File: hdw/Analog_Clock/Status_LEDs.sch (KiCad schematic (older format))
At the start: 35 parts

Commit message: More schematic work
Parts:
- removed U? (x7): 74LVC1G97, Package_TO_SOT_SMD:SOT-363_SC-70-6, symbol Custom_Library:74LVC1G97_Power_NOT
- added U? (x7): 74LVC1G06, TO_SOT_Packages_SMD:SOT-353_SC-70-5, symbol Custom_Library:74LVC1G06_Power
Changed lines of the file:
@@
 EESchema Schematic File Version 4
+LIBS:Analog_Clock-cache
 EELAYER 30 0
 EELAYER END
@@
 $EndComp
 $Comp
-L Custom_Library:74LVC1G97_Power_NOT U?
-U 1 1 5E499235
+L Custom_Library:74LVC1G06_Power U?
+U 1 1 5E9D80F8
 P 2400 2220
-F 0 "U?" H 2460 2370 50  0000 L CNN
-F 1 "74LVC1G97" H 2460 2070 50  0000 L CNN
-F 2 "Package_TO_SOT_SMD:SOT-363_SC-70-6" H 2450 2220 50  0001 C CNN
-F 3 "http://www.ti.com/lit/ds/symlink/sn74lvc1g97.pdf" H 2450 2220 50  0001 C CNN
-F 4 "296-15582-1-ND" H 2400 2220 50  0001 C CNN "Digi-Key PN"
+F 0 "U?" H 2500 2370 50  0000 L CNN
+F 1 "74LVC1G06" H 2500 2120 50  0000 L CNN
+F 2 "TO_SOT_Packages_SMD:SOT-353_SC-70-5" H 2400 2270 50  0001 C CNN
+F 3 "http://www.ti.com/lit/ds/symlink/sn74lvc1g06.pdf" H 2400 2220 50  0001 C CNN
+F 4 "296-8484-1-ND" H 2400 2220 50  0001 C CNN "Digi-Key PN"
 	1    2400 2220
 	1    0    0    -1
 $EndComp
 $Comp
-L Custom_Library:74LVC1G97_Power_NOT U?
-U 1 1 5E499F9B
+L Custom_Library:74LVC1G06_Power U?
+U 1 1 5E9DA040
 P 4400 2220
-F 0 "U?" H 4460 2370 50  0000 L CNN
-F 1 "74LVC1G97" H 4460 2070 50  0000 L CNN
-F 2 "Package_TO_SOT_SMD:SOT-363_SC-70-6" H 4450 2220 50  0001 C CNN
-F 3 "http://www.ti.com/lit/ds/symlink/sn74lvc1g97.pdf" H 4450 2220 50  0001 C CNN
-F 4 "296-15582-1-ND" H 4400 2220 50  0001 C CNN "Digi-Key PN"
+F 0 "U?" H 4500 2370 50  0000 L CNN
+F 1 "74LVC1G06" H 4500 2120 50  0000 L CNN
+F 2 "TO_SOT_Packages_SMD:SOT-353_SC-70-5" H 4400 2270 50  0001 C CNN
+F 3 "http://www.ti.com/lit/ds/symlink/sn74lvc1g06.pdf" H 4400 2220 50  0001 C CNN
+F 4 "296-8484-1-ND" H 4400 2220 50  0001 C CNN "Digi-Key PN"
 	1    4400 2220
 	1    0    0    -1
 $EndComp
 $Comp
-L Custom_Library:74LVC1G97_Power_NOT U?
-U 1 1 5E49A9B3
+L Custom_Library:74LVC1G06_Power U?
+U 1 1 5E9DA915
 P 6400 2220
-F 0 "U?" H 6460 2370 50  0000 L CNN
-F 1 "74LVC1G97" H 6460 2070 50  0000 L CNN
-F 2 "Package_TO_SOT_SMD:SOT-363_SC-70-6" H 6450 2220 50  0001 C CNN
-F 3 "http://www.ti.com/lit/ds/symlink/sn74lvc1g97.pdf" H 6450 2220 50  0001 C CNN
-F 4 "296-15582-1-ND" H 6400 2220 50  0001 C CNN "Digi-Key PN"
+F 0 "U?" H 6500 2370 50  0000 L CNN
+F 1 "74LVC1G06" H 6500 2120 50  0000 L CNN
+F 2 "TO_SOT_Packages_SMD:SOT-353_SC-70-5" H 6400 2270 50  0001 C CNN
+F 3 "http://www.ti.com/lit/ds/symlink/sn74lvc1g06.pdf" H 6400 2220 50  0001 C CNN
+F 4 "296-8484-1-ND" H 6400 2220 50  0001 C CNN "Digi-Key PN"
 	1    6400 2220
 	1    0    0    -1
 $EndComp
 $Comp
-L Custom_Library:74LVC1G97_Power_NOT U?
-U 1 1 5E49B430
+L Custom_Library:74LVC1G06_Power U?
+U 1 1 5E9DB45A
 P 8400 2220
-F 0 "U?" H 8460 2370 50  0000 L CNN
-F 1 "74LVC1G97" H 8460 2070 50  0000 L CNN
-F 2 "Package_TO_SOT_SMD:SOT-363_SC-70-6" H 8450 2220 50  0001 C CNN
-F 3 "http://www.ti.com/lit/ds/symlink/sn74lvc1g97.pdf" H 8450 2220 50  0001 C CNN
-F 4 "296-15582-1-ND" H 8400 2220 50  0001 C CNN "Digi-Key PN"
+F 0 "U?" H 8500 2370 50  0000 L CNN
+F 1 "74LVC1G06" H 8500 2120 50  0000 L CNN
+F 2 "TO_SOT_Packages_SMD:SOT-353_SC-70-5" H 8400 2270 50  0001 C CNN
+F 3 "http://www.ti.com/lit/ds/symlink/sn74lvc1g06.pdf" H 8400 2220 50  0001 C CNN
+F 4 "296-8484-1-ND" H 8400 2220 50  0001 C CNN "Digi-Key PN"
 	1    8400 2220
 	1    0    0    -1
 $EndComp
 $Comp
-L Custom_Library:74LVC1G97_Power_NOT U?
-U 1 1 5E49BF58
+L Custom_Library:74LVC1G06_Power U?
+U 1 1 5E9DBF5D
 P 6400 4220
-F 0 "U?" H 6460 4370 50  0000 L CNN
-F 1 "74LVC1G97" H 6460 4070 50  0000 L CNN
-F 2 "Package_TO_SOT_SMD:SOT-363_SC-70-6" H 6450 4220 50  0001 C CNN
-F 3 "http://www.ti.com/lit/ds/symlink/sn74lvc1g97.pdf" H 6450 4220 50  0001 C CNN
-F 4 "296-15582-1-ND" H 6400 4220 50  0001 C CNN "Digi-Key PN"
+F 0 "U?" H 6500 4370 50  0000 L CNN
+F 1 "74LVC1G06" H 6500 4120 50  0000 L CNN
+F 2 "TO_SOT_Packages_SMD:SOT-353_SC-70-5" H 6400 4270 50  0001 C CNN
+F 3 "http://www.ti.com/lit/ds/symlink/sn74lvc1g06.pdf" H 6400 4220 50  0001 C CNN
+F 4 "296-8484-1-ND" H 6400 4220 50  0001 C CNN "Digi-Key PN"
 	1    6400 4220
 	1    0    0    -1
 $EndComp
 $Comp
-L Custom_Library:74LVC1G97_Power_NOT U?
-U 1 1 5E49CDEC
+L Custom_Library:74LVC1G06_Power U?
+U 1 1 5E9DCA66
 P 4400 4220
-F 0 "U?" H 4460 4370 50  0000 L CNN
-F 1 "74LVC1G97" H 4460 4070 50  0000 L CNN
-F 2 "Package_TO_SOT_SMD:SOT-363_SC-70-6" H 4450 4220 50  0001 C CNN
-F 3 "http://www.ti.com/lit/ds/symlink/sn74lvc1g97.pdf" H 4450 4220 50  0001 C CNN
-F 4 "296-15582-1-ND" H 4400 4220 50  0001 C CNN "Digi-Key PN"
+F 0 "U?" H 4500 4370 50  0000 L CNN
+F 1 "74LVC1G06" H 4500 4120 50  0000 L CNN
+F 2 "TO_SOT_Packages_SMD:SOT-353_SC-70-5" H 4400 4270 50  0001 C CNN
+F 3 "http://www.ti.com/lit/ds/symlink/sn74lvc1g06.pdf" H 4400 4220 50  0001 C CNN
+F 4 "296-8484-1-ND" H 4400 4220 50  0001 C CNN "Digi-Key PN"
 	1    4400 4220
 	1    0    0    -1
 $EndComp
 $Comp
-L Custom_Library:74LVC1G97_Power_NOT U?
-U 1 1 5E49D6D6
+L Custom_Library:74LVC1G06_Power U?
+U 1 1 5E9DD4E5
 P 2400 4220
-F 0 "U?" H 2460 4370 50  0000 L CNN
-F 1 "74LVC1G97" H 2460 4070 50  0000 L CNN
-F 2 "Package_TO_SOT_SMD:SOT-363_SC-70-6" H 2450 4220 50  0001 C CNN
-F 3 "http://www.ti.com/lit/ds/symlink/sn74lvc1g97.pdf" H 2450 4220 50  0001 C CNN
-F 4 "296-15582-1-ND" H 2400 4220 50  0001 C CNN "Digi-Key PN"
+F 0 "U?" H 2500 4370 50  0000 L CNN
+F 1 "74LVC1G06" H 2500 4120 50  0000 L CNN
+F 2 "TO_SOT_Packages_SMD:SOT-353_SC-70-5" H 2400 4270 50  0001 C CNN
+F 3 "http://www.ti.com/lit/ds/symlink/sn74lvc1g06.pdf" H 2400 4220 50  0001 C CNN
+F 4 "296-8484-1-ND" H 2400 4220 50  0001 C CNN "Digi-Key PN"
 	1    2400 4220
 	1    0    0    -1

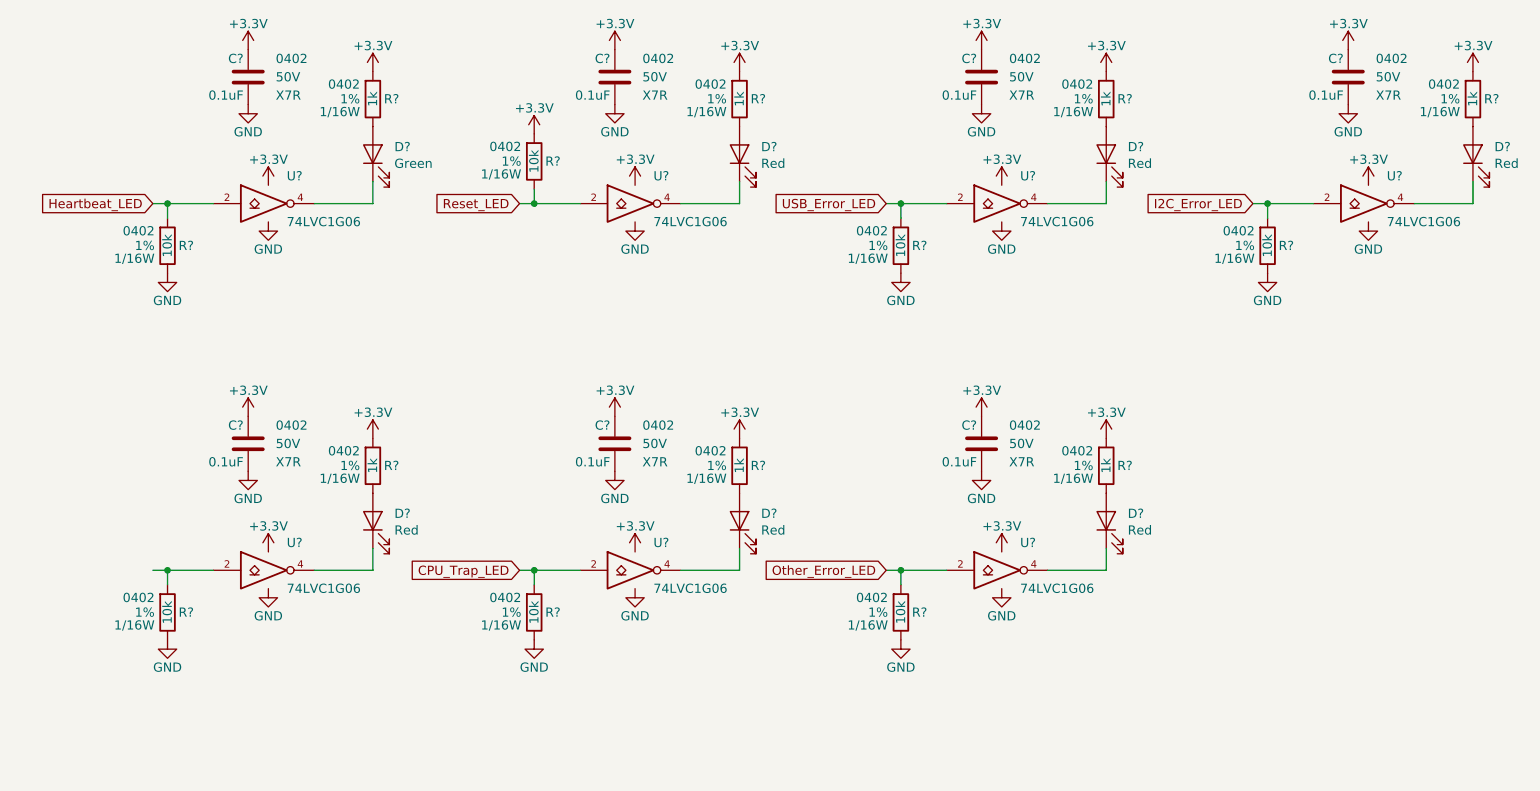
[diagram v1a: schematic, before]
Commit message: More sch work
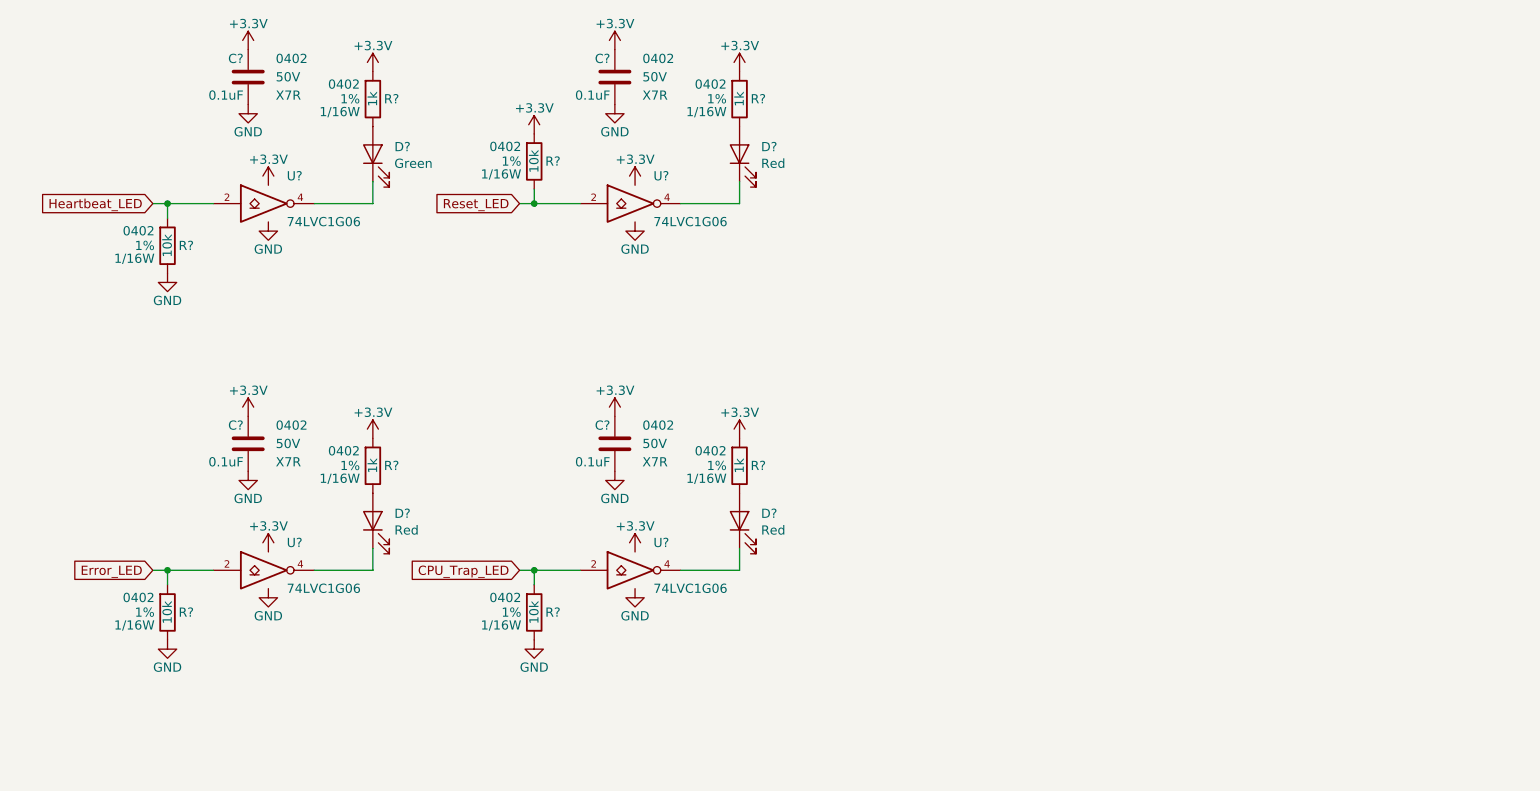
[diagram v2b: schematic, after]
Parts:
- removed C? (x3): 0.1uF, Capacitors_SMD:C_0402, symbol Custom_Library:C_Custom
- removed D? (x3): Red, symbol Device:LED
- removed R? (x3): 1k, Resistors_SMD:R_0402, symbol Custom_Library:R_Custom
- removed R? (x3): 10k, Resistors_SMD:R_0402, symbol Custom_Library:R_Custom
- removed U? (x3): 74LVC1G06, TO_SOT_Packages_SMD:SOT-353_SC-70-5, symbol Custom_Library:74LVC1G06_Power
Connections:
- net labels added: Error_LED
- net labels removed: I2C_Error_LED, Other_Error_LED, USB_Error_LED
- wire segments 35 -> 20

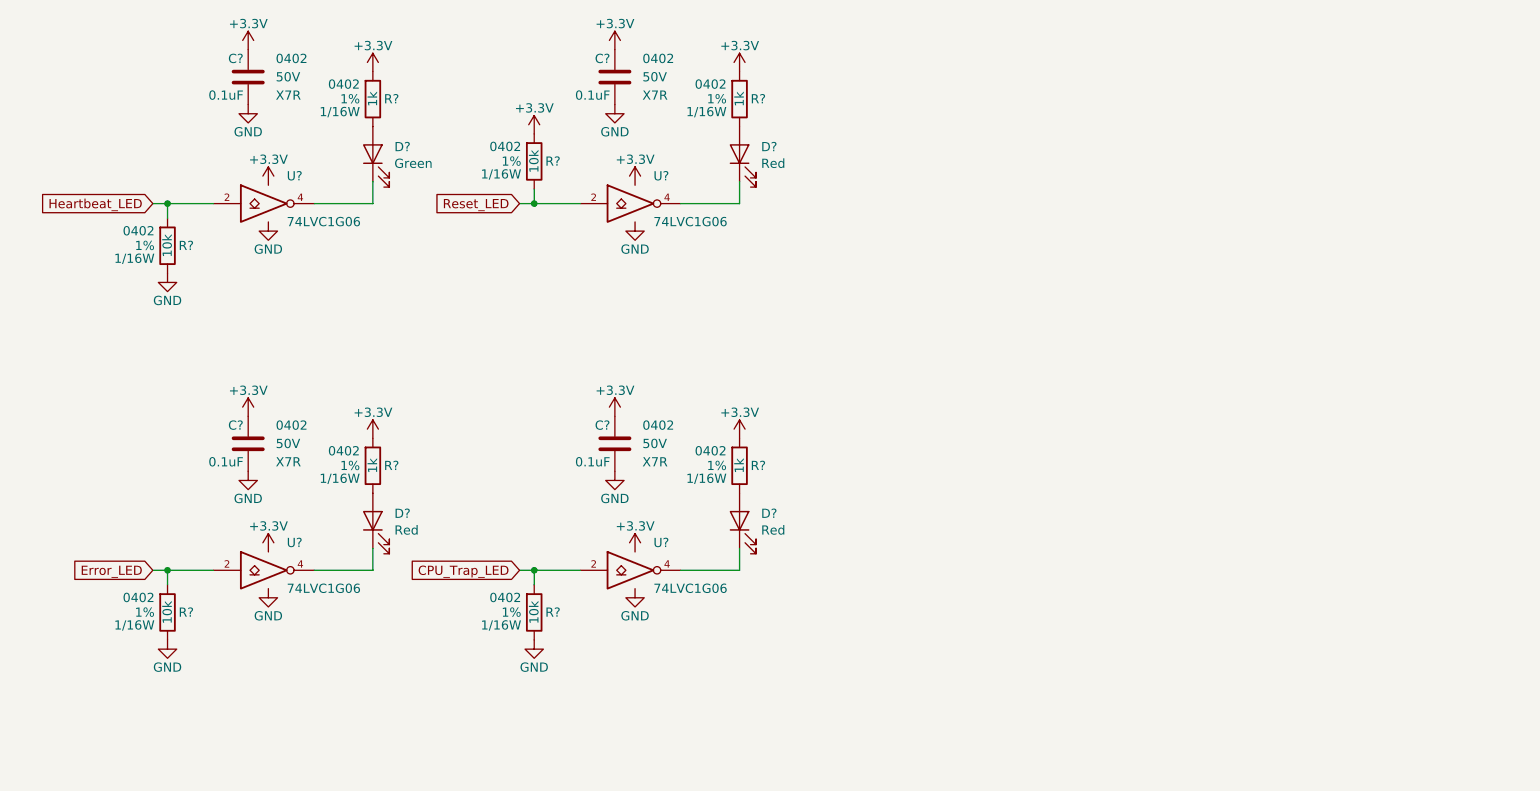
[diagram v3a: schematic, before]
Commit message: more analog work, added some more sch stuff
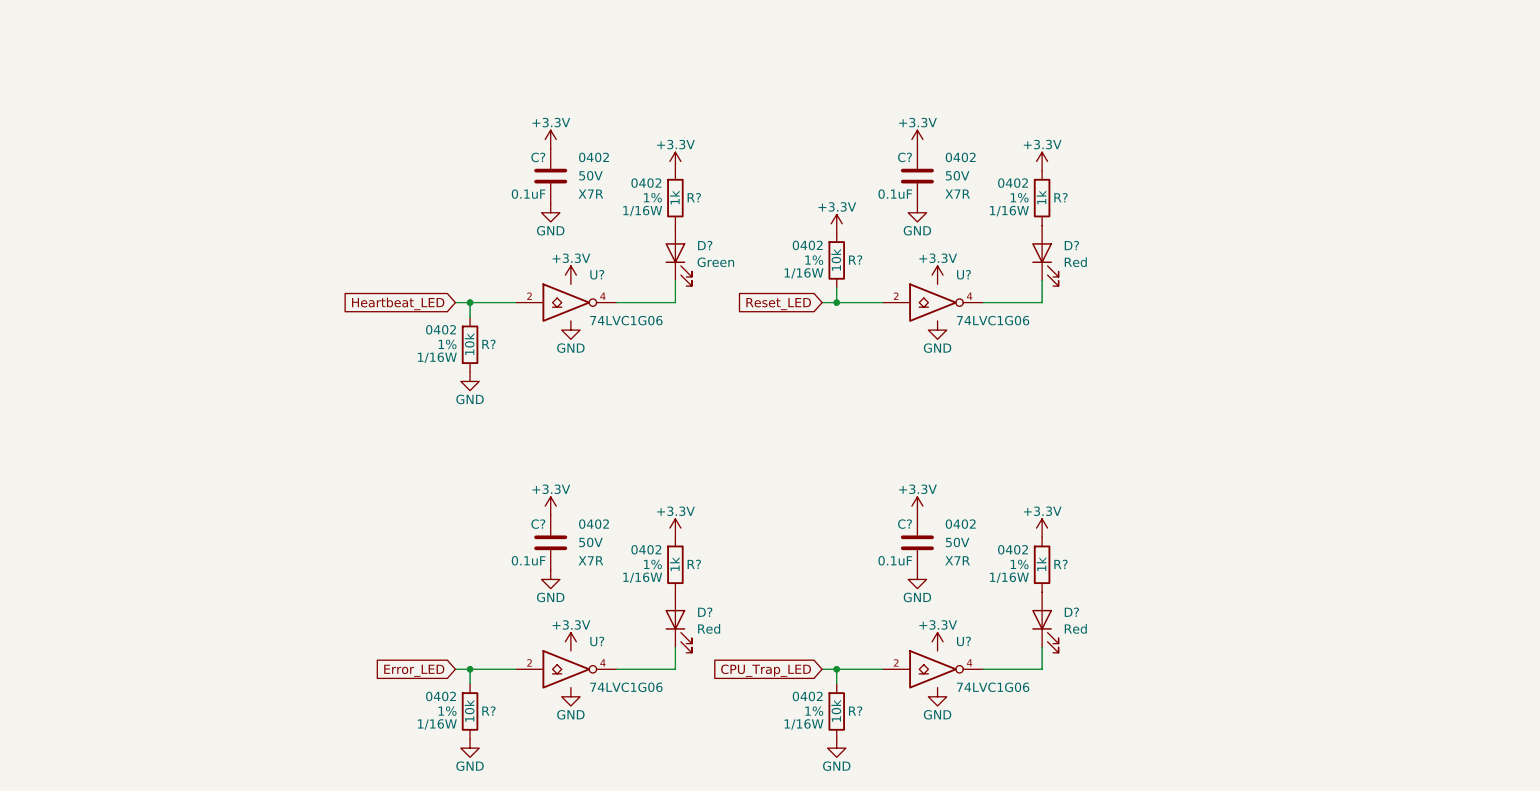
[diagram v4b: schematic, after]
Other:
- moved on the sheet: C?, D?, R?, U?

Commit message: big sch push
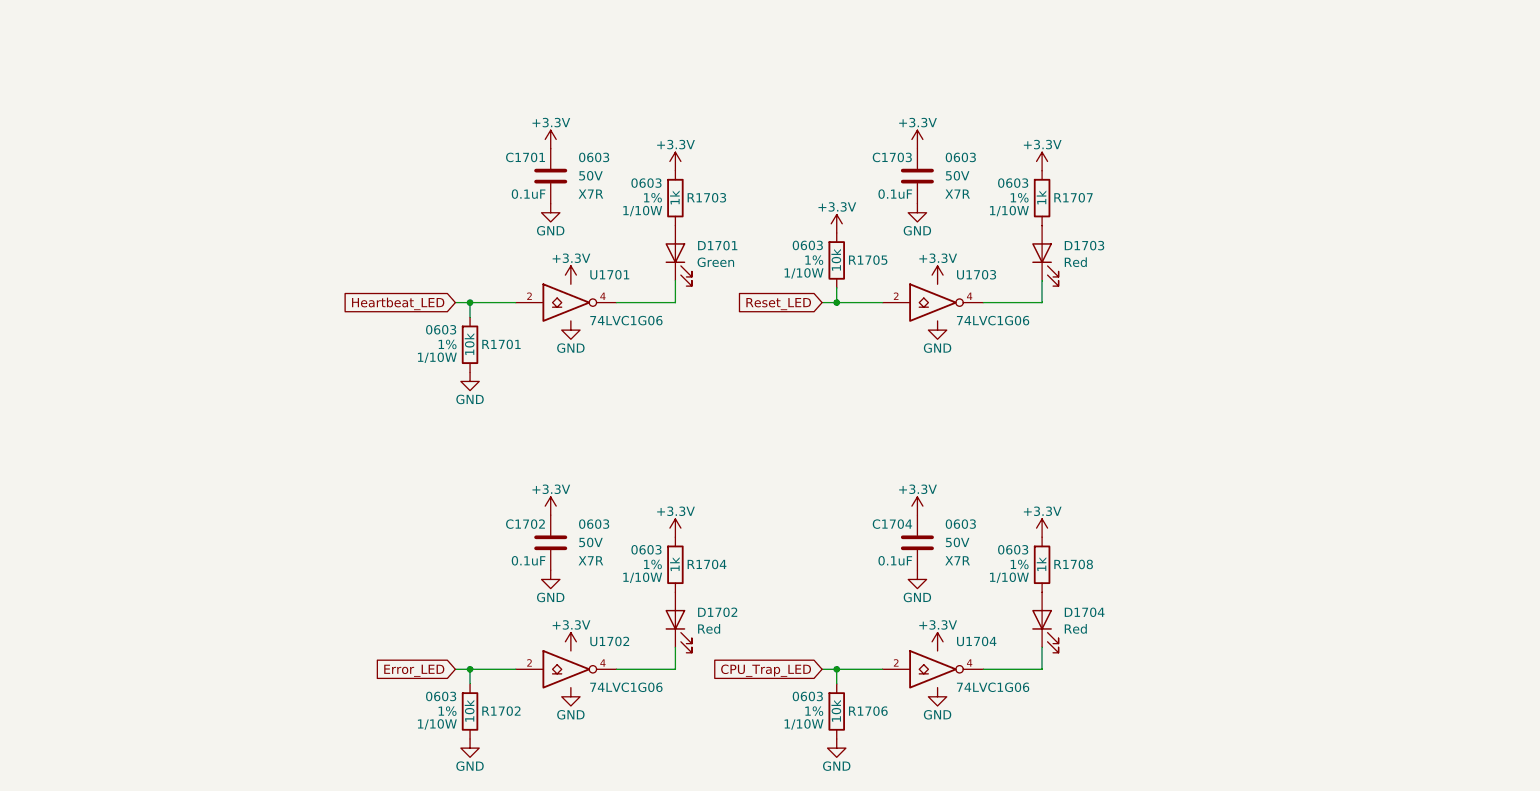
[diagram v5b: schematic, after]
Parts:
- C1701, C1702, C1703, C1704: renamed from C?; footprint Capacitors_SMD:C_0402 -> Capacitors_SMD:C_0603; Digi-Key PN 490-10701-1-ND -> 399-7845-1-ND; display_footprint 0402 -> 0603
- D1701: renamed from D?; footprint (none) -> LEDs:LED_0603; Digi-Key PN (none) -> 754-1121-1-ND
- D1702, D1703, D1704: renamed from D?; footprint (none) -> LEDs:LED_0603; Digi-Key PN (none) -> 754-1117-1-ND
- R1701, R1702, R1705, R1706: renamed from R?; footprint Resistors_SMD:R_0402 -> Resistors_SMD:R_0603; Digi-Key PN RMCF0402FT10K0CT-ND -> (none); Wattage 1/16W -> 1/10W; display_footprint 0402 -> 0603
- R1703, R1704, R1707, R1708: renamed from R?; footprint Resistors_SMD:R_0402 -> Resistors_SMD:R_0603; Digi-Key PN 541-1.00KLCT-ND -> (none); Wattage 1/16W -> 1/10W; display_footprint 0402 -> 0603
- gave numbers to parts that had none: 4

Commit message: Much more schematic progress
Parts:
- R1701, R1702, R1705, R1706: Digi-Key PN (none) -> YAG2321CT-ND
- R1703, R1704, R1707, R1708: Digi-Key PN (none) -> 311-1.00KHRCT-ND
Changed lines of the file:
@@
 encoding utf-8
 Sheet 17 25
-Title ""
-Date ""
-Rev ""
-Comp ""
+Title "Analog Clock"
+Date "2020-08-15"
+Rev "A"
+Comp "Drew Maatman"
 Comment1 ""
 Comment2 ""
@@
 F 5 "1%" H 4690 2190 50  0000 L CNN "Tolerance"
 F 6 "1/10W" H 4690 2120 50  0000 L CNN "Wattage"
-F 7 "" H 4920 2590 60  0001 C CNN "Digi-Key PN"
+F 7 "311-1.00KHRCT-ND" H 4920 2590 60  0001 C CNN "Digi-Key PN"
 	1    4620 2190
 	-1   0    0    -1
@@
 F 5 "1%" H 3570 2990 50  0000 L CNN "Tolerance"
 F 6 "1/10W" H 3570 2920 50  0000 L CNN "Wattage"
-F 7 "" H 3500 2990 50  0001 C CNN "Digi-Key PN"
+F 7 "YAG2321CT-ND" H 3500 2990 50  0001 C CNN "Digi-Key PN"
 	1    3500 2990
 	-1   0    0    -1
@@
 F 5 "1%" H 6690 2190 50  0000 L CNN "Tolerance"
 F 6 "1/10W" H 6690 2120 50  0000 L CNN "Wattage"
-F 7 "" H 6920 2590 60  0001 C CNN "Digi-Key PN"
+F 7 "311-1.00KHRCT-ND" H 6920 2590 60  0001 C CNN "Digi-Key PN"
 	1    6620 2190
 	-1   0    0    -1
@@
 F 5 "1%" H 5570 2530 50  0000 L CNN "Tolerance"
 F 6 "1/10W" H 5570 2460 50  0000 L CNN "Wattage"
-F 7 "" H 5500 2530 50  0001 C CNN "Digi-Key PN"
+F 7 "YAG2321CT-ND" H 5500 2530 50  0001 C CNN "Digi-Key PN"
 	1    5500 2530
 	-1   0    0    -1
@@
 F 5 "1%" H 4690 4190 50  0000 L CNN "Tolerance"
 F 6 "1/10W" H 4690 4120 50  0000 L CNN "Wattage"
-F 7 "" H 4920 4590 60  0001 C CNN "Digi-Key PN"
+F 7 "311-1.00KHRCT-ND" H 4920 4590 60  0001 C CNN "Digi-Key PN"
 	1    4620 4190
 	-1   0    0    -1
@@
 F 5 "1%" H 3570 4990 50  0000 L CNN "Tolerance"
 F 6 "1/10W" H 3570 4920 50  0000 L CNN "Wattage"
-F 7 "" H 3500 4990 50  0001 C CNN "Digi-Key PN"
+F 7 "YAG2321CT-ND" H 3500 4990 50  0001 C CNN "Digi-Key PN"
 	1    3500 4990
 	-1   0    0    -1
@@
 F 5 "1%" H 6690 4190 50  0000 L CNN "Tolerance"
 F 6 "1/10W" H 6690 4120 50  0000 L CNN "Wattage"
-F 7 "" H 6920 4590 60  0001 C CNN "Digi-Key PN"
+F 7 "311-1.00KHRCT-ND" H 6920 4590 60  0001 C CNN "Digi-Key PN"
 	1    6620 4190
 	-1   0    0    -1
@@
 F 5 "1%" H 5570 4990 50  0000 L CNN "Tolerance"
 F 6 "1/10W" H 5570 4920 50  0000 L CNN "Wattage"
-F 7 "" H 5500 4990 50  0001 C CNN "Digi-Key PN"
+F 7 "YAG2321CT-ND" H 5500 4990 50  0001 C CNN "Digi-Key PN"
 	1    5500 4990
 	-1   0    0    -1
